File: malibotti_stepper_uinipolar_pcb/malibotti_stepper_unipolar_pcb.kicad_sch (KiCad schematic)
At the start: 34 parts, among them J1 Stepper 1, J2 Stepper 2, J3 Servo, J4 I2C, J5 USB_C_Receptacle_USB2.0_16P, J6 Serial, SW1 RST, SW2 MicroSwitchLeft, SW3 MicroSwitchRight, SW8 BTN, U1 TBD62783A, U3 AMS1117, U5 ESP32-S3-MINI-1

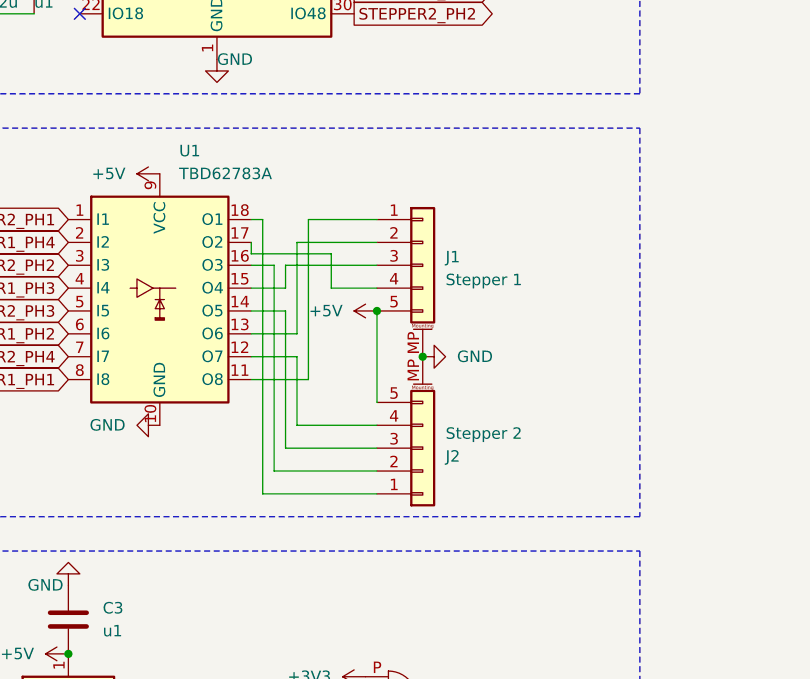
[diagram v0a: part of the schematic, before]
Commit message: Varions
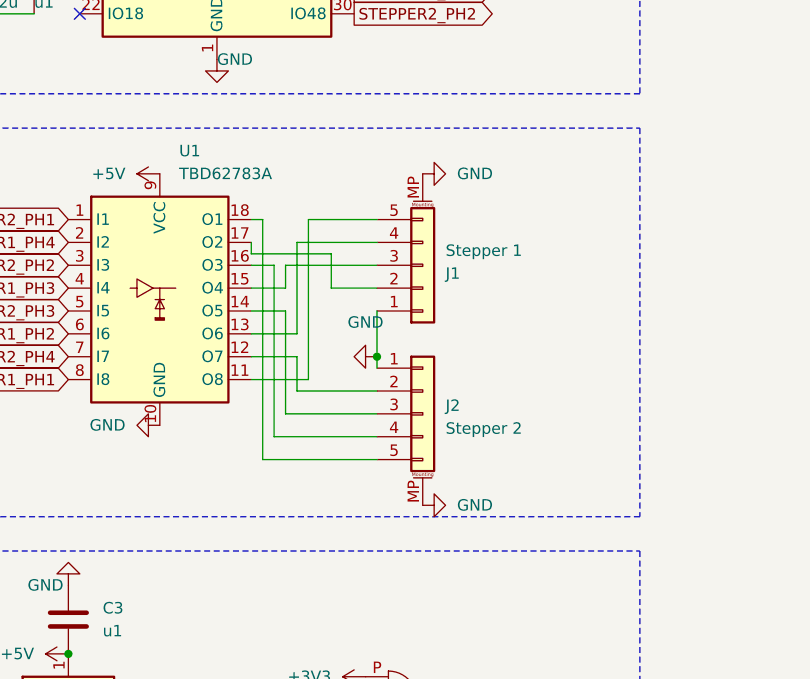
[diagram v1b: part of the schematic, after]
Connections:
- net +5V: no longer J1.5 (Pin_5), J2.5 (Pin_5)
- net GND: now also J1.1 (Pin_1), J2.1 (Pin_1)
- net at U1.18 (O1): now also J2.5 (Pin_5); no longer J2.1 (Pin_1)
- net at J2.2 (Pin_2): now also U1.12 (O7); no longer U1.16 (O3)
- net at J2.4 (Pin_4): now also U1.16 (O3); no longer U1.12 (O7)
- net at U1.11 (O8): now also J1.5 (Pin_5); no longer J1.1 (Pin_1)
- net at U1.13 (O6): now also J1.4 (Pin_4); no longer J1.2 (Pin_2)
- net at U1.17 (O2): now also J1.2 (Pin_2); no longer J1.4 (Pin_4)
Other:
- moved on the sheet: J1
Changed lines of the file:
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@@
 	)
 	(junction
-		(at 67.31 110.49)
-		(diameter 0)
-		(color 0 0 0 0)
-	)
-	(junction
 		(at 33.02 148.59)
 		(diameter 0)
@@
 	)
 	(junction
-		(at 55.88 179.07)
+		(at 67.31 115.57)
 		(diameter 0)
 		(color 0 0 0 0)
 	)
 	(junction
-		(at 198.12 30.48)
+		(at 55.88 179.07)
 		(diameter 0)
 		(color 0 0 0 0)
 	)
 	(junction
-		(at 72.39 115.57)
+		(at 198.12 30.48)
 		(diameter 0)
 		(color 0 0 0 0)
@@
 	(wire
 		(pts
-			(xy 67.31 128.27) (xy 55.88 128.27)
+			(xy 67.31 124.46) (xy 55.88 124.46)
 		)
 		(stroke
@@
 	(wire
 		(pts
-			(xy 55.88 128.27) (xy 55.88 105.41)
+			(xy 55.88 124.46) (xy 55.88 105.41)
 		)
 		(stroke
@@
 	(wire
 		(pts
-			(xy 57.15 125.73) (xy 57.15 110.49)
+			(xy 57.15 121.92) (xy 57.15 110.49)
 		)
 		(stroke
@@
 	(wire
 		(pts
-			(xy 67.31 130.81) (xy 54.61 130.81)
+			(xy 67.31 127) (xy 54.61 127)
 		)
 		(stroke
@@
 	(wire
 		(pts
+			(xy 67.31 115.57) (xy 67.31 116.84)
+		)
+		(stroke
+			(width 0)
+			(type default)
+		)
+	)
+	(wire
+		(pts
 			(xy 58.42 102.87) (xy 58.42 113.03)
 		)
@@
 	(wire
 		(pts
-			(xy 54.61 130.81) (xy 54.61 100.33)
+			(xy 54.61 127) (xy 54.61 100.33)
 		)
 		(stroke
@@
 	(wire
 		(pts
-			(xy 67.31 110.49) (xy 67.31 120.65)
+			(xy 67.31 110.49) (xy 67.31 115.57)
 		)
 		(stroke
@@
 	(wire
 		(pts
-			(xy 58.42 123.19) (xy 58.42 115.57)
+			(xy 58.42 119.38) (xy 58.42 115.57)
 		)
 		(stroke
@@
 	(wire
 		(pts
-			(xy 67.31 125.73) (xy 57.15 125.73)
+			(xy 67.31 121.92) (xy 57.15 121.92)
 		)
 		(stroke
@@
 	(wire
 		(pts
-			(xy 67.31 123.19) (xy 58.42 123.19)
+			(xy 67.31 119.38) (xy 58.42 119.38)
 		)
 		(stroke
@@
 	)
 	(symbol
-		(lib_id "power:+5V")
-		(at 67.31 110.49 90)
-		(unit 1)
-		(body_style 1)
-		(exclude_from_sim no)
-		(in_bom yes)
-		(on_board yes)
-		(in_pos_files yes)
-		(dnp no)
-		(fields_autoplaced yes)
-		(property "Reference" "#PWR048"
-			(at 71.12 110.49 0)
-			(hide yes)
-			(show_name no)
-			(do_not_autoplace no)
-			(effects
-				(font
-					(size 1.27 1.27)
-				)
-			)
-		)
-		(property "Value" "+5V"
-			(at 63.5 110.4899 90)
-			(show_name no)
-			(do_not_autoplace no)
-			(effects
-				(font
-					(size 1.27 1.27)
-				)
-				(justify left)
-			)
-		)
-		(property "Footprint" ""
-			(at 67.31 110.49 0)
-			(hide yes)
-			(show_name no)
-			(do_not_autoplace no)
-			(effects
-				(font
-					(size 1.27 1.27)
-				)
-			)
-		)
-		(property "Datasheet" ""
-			(at 67.31 110.49 0)
-			(hide yes)
-			(show_name no)
-			(do_not_autoplace no)
-			(effects
-				(font
-					(size 1.27 1.27)
-				)
-			)
-		)
-		(property "Description" "Power symbol creates a global label with name \"+5V\""
-			(at 67.31 110.49 0)
-			(hide yes)
-			(show_name no)
-			(do_not_autoplace no)
-			(effects
-				(font
-					(size 1.27 1.27)
-				)
-			)
-		)
-		(pin "1"
-		)
-		(instances
-			(project "malibotti_stepper_unipolar_pcb"
-				(path "/e3c0928e-588c-4cab-a021-dc1d90fa1136"
-					(reference "#PWR048")
-					(unit 1)
-				)
-			)
-		)
-	)
-	(symbol
 		(lib_id "Connector_Generic:Conn_01x04")
 		(at 86.36 29.21 0)
@@
 	(symbol
 		(lib_id "Connector_Generic_MountingPin:Conn_01x05_MountingPin")
-		(at 72.39 125.73 0)
-		(mirror x)
+		(at 72.39 121.92 0)
 		(unit 1)
 		(body_style 1)
@@
 		(dnp no)
 		(property "Reference" "J2"
-			(at 74.93 126.6445 0)
+			(at 74.93 121.0055 0)
 			(show_name no)
 			(do_not_autoplace no)
@@
 		)
 		(property "Value" "Stepper 2"
-			(at 74.93 124.1045 0)
+			(at 74.93 123.5455 0)
 			(show_name no)
 			(do_not_autoplace no)
@@
 		)
 		(property "Footprint" "liebler_CONN:JST_XH_5P_SMD"
-			(at 72.39 125.73 0)
+			(at 72.39 121.92 0)
 			(hide yes)
 			(show_name no)
@@
 		)
 		(property "Datasheet" ""
-			(at 72.39 125.73 0)
+			(at 72.39 121.92 0)
 			(hide yes)
 			(show_name no)
@@
 		)
 		(property "Description" "Generic connectable mounting pin connector, single row, 01x05, script generated (kicad-library-utils/schlib/autogen/connector/)"
-			(at 72.39 125.73 0)
+			(at 72.39 121.92 0)
 			(hide yes)
 			(show_name no)
@@
 	)
 	(symbol
+		(lib_id "power:GND")
+		(at 72.39 132.08 90)
+		(unit 1)
+		(body_style 1)
+		(exclude_from_sim no)
+		(in_bom yes)
+		(on_board yes)
+		(in_pos_files yes)
+		(dnp no)
+		(fields_autoplaced yes)
+		(property "Reference" "#PWR053"
+			(at 78.74 132.08 0)
+			(hide yes)
+			(show_name no)
+			(do_not_autoplace no)
+			(effects
+				(font
+					(size 1.27 1.27)
+				)
+			)
+		)
+		(property "Value" "GND"
+			(at 76.2 132.0799 90)
+			(show_name no)
+			(do_not_autoplace no)
+			(effects
+				(font
+					(size 1.27 1.27)
+				)
+				(justify right)
+			)
+		)
+		(property "Footprint" ""
+			(at 72.39 132.08 0)
+			(hide yes)
+			(show_name no)
+			(do_not_autoplace no)
+			(effects
+				(font
+					(size 1.27 1.27)
+				)
+			)
+		)
+		(property "Datasheet" ""
+			(at 72.39 132.08 0)
+			(hide yes)
+			(show_name no)
+			(do_not_autoplace no)
+			(effects
+				(font
+					(size 1.27 1.27)
+				)
+			)
+		)
+		(property "Description" "Power symbol creates a global label with name \"GND\" , ground"
+			(at 72.39 132.08 0)
+			(hide yes)
+			(show_name no)
+			(do_not_autoplace no)
+			(effects
+				(font
+					(size 1.27 1.27)
+				)
+			)
+		)
+		(pin "1"
+		)
+		(instances
+			(project "malibotti_stepper_unipolar_pcb"
+				(path "/e3c0928e-588c-4cab-a021-dc1d90fa1136"
+					(reference "#PWR053")
+					(unit 1)
+				)
+			)
+		)
+	)
+	(symbol
 		(lib_id "Device:C")
 		(at 46.99 182.88 0)
@@
 		(lib_id "Connector_Generic_MountingPin:Conn_01x05_MountingPin")
 		(at 72.39 105.41 0)
+		(mirror x)
 		(unit 1)
 		(body_style 1)
@@
 		(in_pos_files yes)
 		(dnp no)
-		(fields_autoplaced yes)
 		(property "Reference" "J1"
-			(at 74.93 104.4955 0)
+			(at 74.93 106.3245 0)
 			(show_name no)
 			(do_not_autoplace no)
@@
 		)
 		(property "Value" "Stepper 1"
-			(at 74.93 107.0355 0)
+			(at 74.93 103.7845 0)
 			(show_name no)
 			(do_not_autoplace no)
@@
 	(symbol
 		(lib_id "power:GND")
+		(at 72.39 95.25 90)
+		(unit 1)
+		(body_style 1)
+		(exclude_from_sim no)
+		(in_bom yes)
+		(on_board yes)
+		(in_pos_files yes)
+		(dnp no)
+		(fields_autoplaced yes)
+		(property "Reference" "#PWR050"
+			(at 78.74 95.25 0)
+			(hide yes)
+			(show_name no)
+			(do_not_autoplace no)
+			(effects
+				(font
+					(size 1.27 1.27)
+				)
+			)
+		)
+		(property "Value" "GND"
+			(at 76.2 95.2499 90)
+			(show_name no)
+			(do_not_autoplace no)
+			(effects
+				(font
+					(size 1.27 1.27)
+				)
+				(justify right)
+			)
+		)
+		(property "Footprint" ""
+			(at 72.39 95.25 0)
+			(hide yes)
+			(show_name no)
+			(do_not_autoplace no)
+			(effects
+				(font
+					(size 1.27 1.27)
+				)
+			)
+		)
+		(property "Datasheet" ""
+			(at 72.39 95.25 0)
+			(hide yes)
+			(show_name no)
+			(do_not_autoplace no)
+			(effects
+				(font
+					(size 1.27 1.27)
+				)
+			)
+		)
+		(property "Description" "Power symbol creates a global label with name \"GND\" , ground"
+			(at 72.39 95.25 0)
+			(hide yes)
+			(show_name no)
+			(do_not_autoplace no)
+			(effects
+				(font
+					(size 1.27 1.27)
+				)
+			)
+		)
+		(pin "1"
+		)
+		(instances
+			(project "malibotti_stepper_unipolar_pcb"
+				(path "/e3c0928e-588c-4cab-a021-dc1d90fa1136"
+					(reference "#PWR050")
+					(unit 1)
+				)
+			)
+		)
+	)
+	(symbol
+		(lib_id "power:GND")
 		(at 21.59 26.67 270)
 		(unit 1)
@@
 	(symbol
 		(lib_id "power:GND")
-		(at 72.39 115.57 90)
+		(at 67.31 115.57 270)
 		(unit 1)
 		(body_style 1)
@@
 		(fields_autoplaced yes)
 		(property "Reference" "#PWR049"
-			(at 78.74 115.57 0)
+			(at 60.96 115.57 0)
 			(hide yes)
 			(show_name no)
@@
 		)
 		(property "Value" "GND"
-			(at 76.2 115.5699 90)
+			(at 66.04 111.76 90)
 			(show_name no)
 			(do_not_autoplace no)
@@
 					(size 1.27 1.27)
 				)
-				(justify right)
 			)
 		)
 		(property "Footprint" ""
-			(at 72.39 115.57 0)
+			(at 67.31 115.57 0)
 			(hide yes)
 			(show_name no)
@@
 		)
 		(property "Datasheet" ""
-			(at 72.39 115.57 0)
+			(at 67.31 115.57 0)
 			(hide yes)
 			(show_name no)
@@
 		)
 		(property "Description" "Power symbol creates a global label with name \"GND\" , ground"
-			(at 72.39 115.57 0)
+			(at 67.31 115.57 0)
 			(hide yes)
 			(show_name no)
